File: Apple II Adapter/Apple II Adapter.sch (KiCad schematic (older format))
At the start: 21 parts, among them J1 IDC_PORT1, J2 IDC_PORT2, M1 Mounting, U1 74HCT04, U2 4066

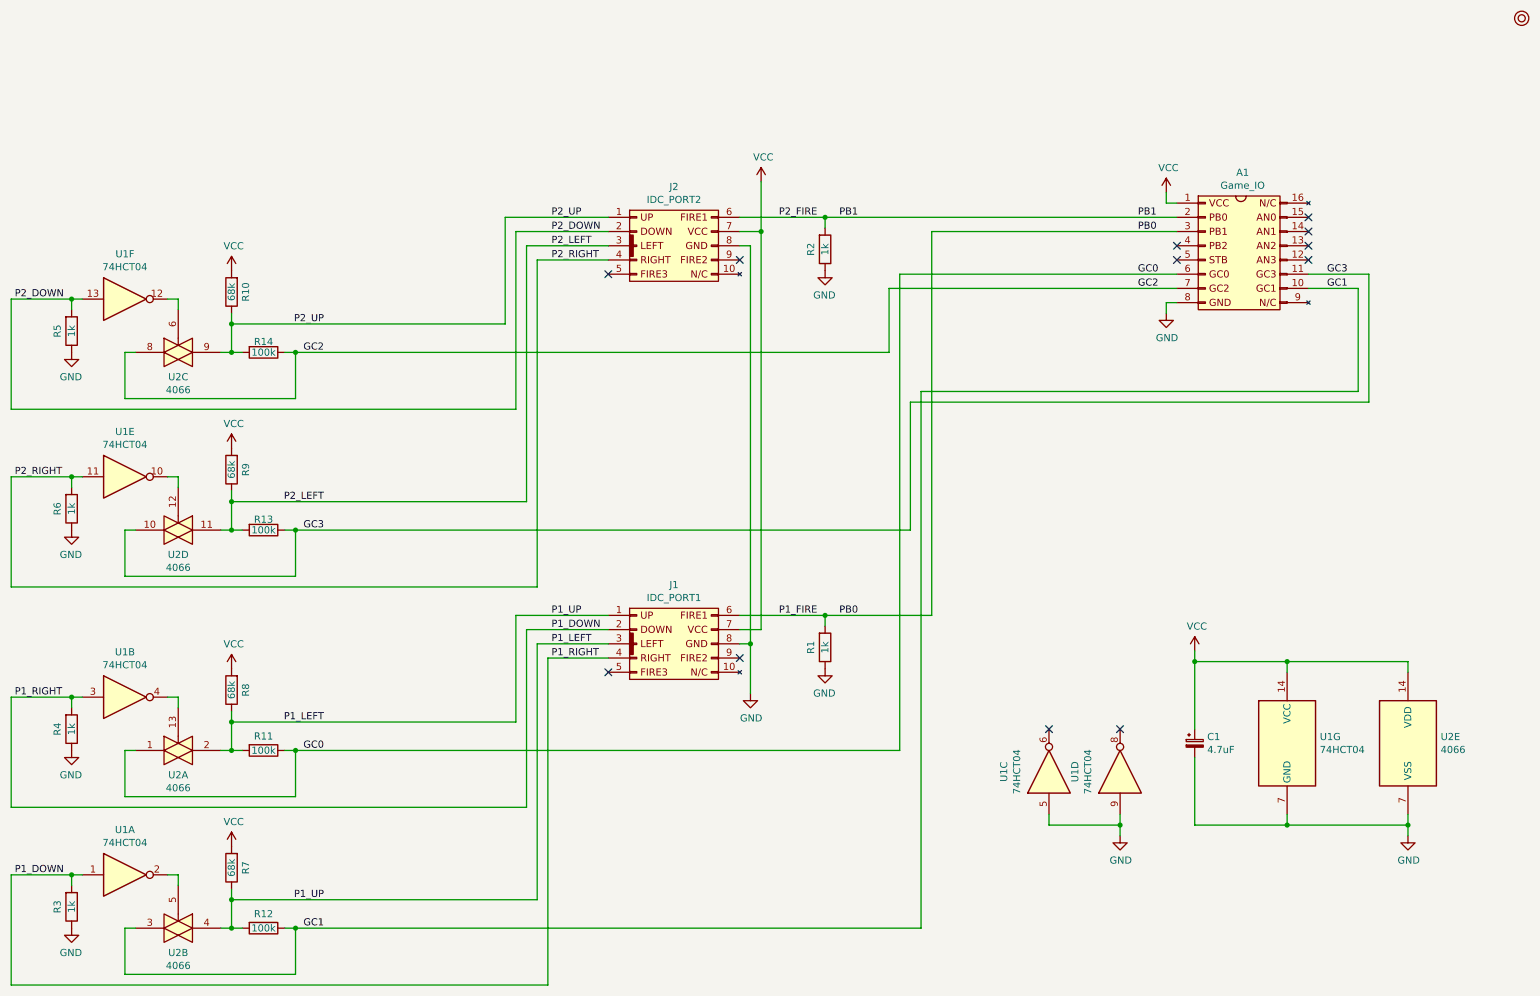
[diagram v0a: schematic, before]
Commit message: Layout routed
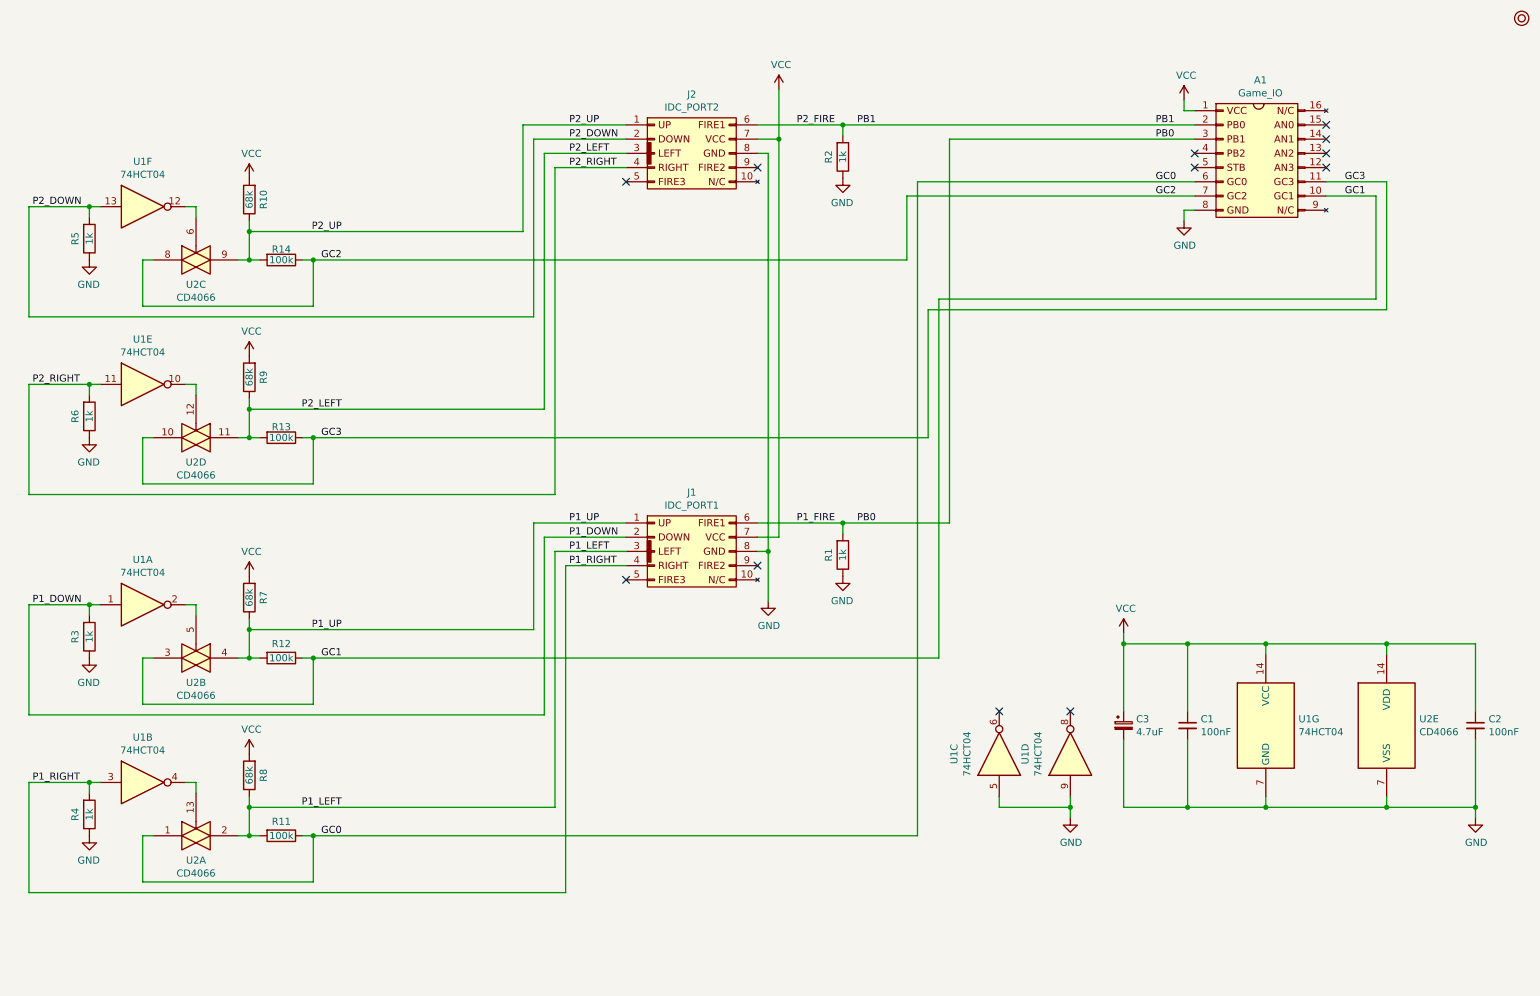
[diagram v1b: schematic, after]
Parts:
- added C1, C2: 100nF, Capacitor_THT:C_Disc_D4.7mm_W2.5mm_P5.00mm, symbol Device:C_Small
- A1: footprint Package_DIP:DIP-16_W7.62mm_Socket_LongPads -> adapter:DIP-16_W7.62mm_Socket_LongPads
- M1: footprint Mounting:M3 -> Mounting:M3_pin
- R5, R6: footprint Resistor_THT:R_Axial_DIN0207_L6.3mm_D2.5mm_P10.16mm_Horizontal -> Resistor_THT:R_Axial_DIN0207_L6.3mm_D2.5mm_P7.62mm_Horizontal
- U2: value 4066 -> CD4066
- renumbered C1 to C3
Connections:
- net GND: now also C1.2, C2.2
- net P1_DOWN: no longer J1.4 (Pin_4), R4.2, U1.3
- net P1_LEFT: no longer J1.1 (Pin_1), R12.2, R7.1, U2.4
- net VCC: now also C1.1, C2.1
- new net P1_RIGHT: J1.4 (Pin_4), R4.2, U1.3
- new net P1_UP: J1.1 (Pin_1), R12.2, R7.1, U2.4
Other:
- moved on the sheet: A1, C3, J1, J2, R1, R10, R11, R12, R13, R14, R2, R3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
